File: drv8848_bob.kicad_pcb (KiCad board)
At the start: 2 copper layers, 21 x 80 mm, 21 parts, among them J1 Conn_01x04_Female, J2 Conn_01x24, J3 Conn_01x04_Female, J4 Conn_01x04_Female, J5 Conn_01x04_Female, U1 DRV8848, U2 DRV8848, U3 DRV8848, U4 DRV8848

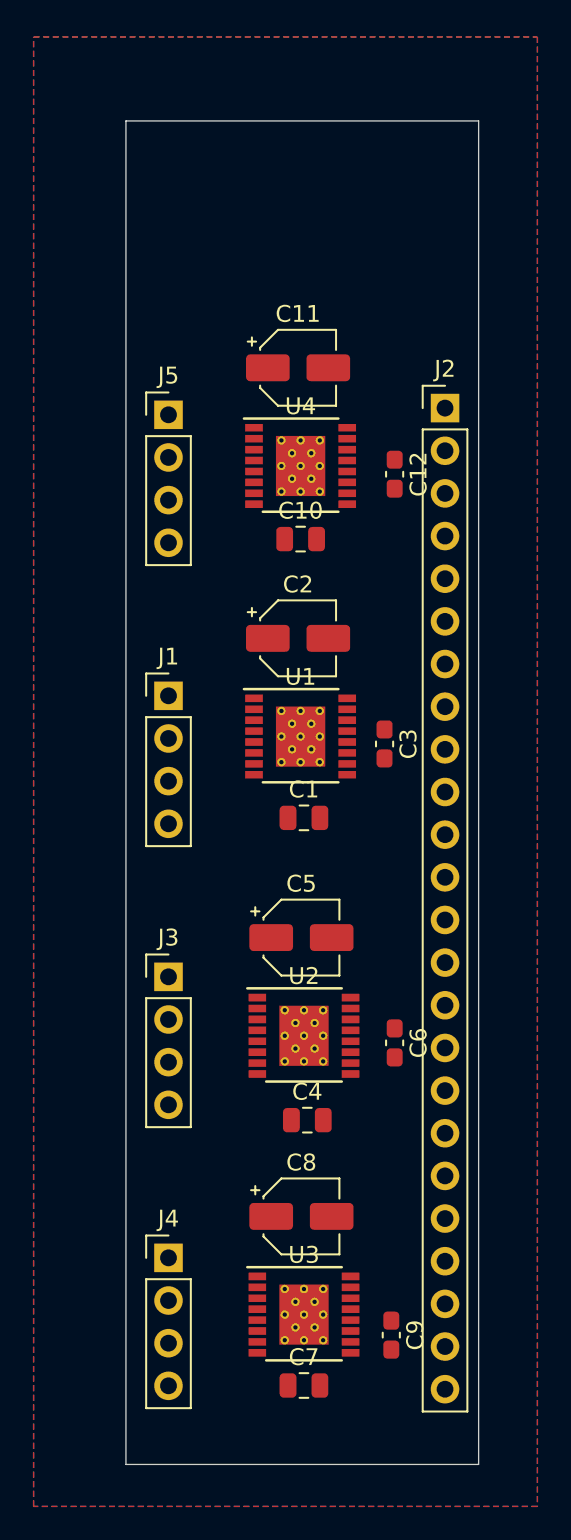
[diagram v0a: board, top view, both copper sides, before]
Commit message: finalish
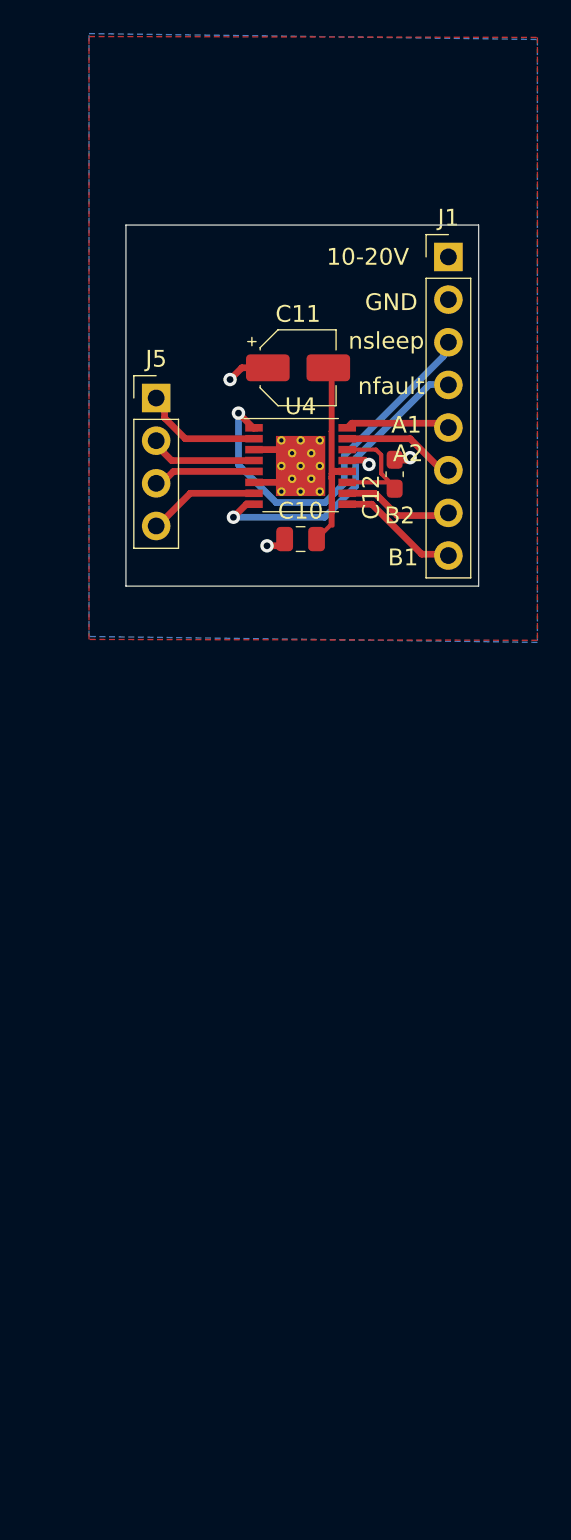
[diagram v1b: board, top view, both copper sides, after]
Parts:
- removed C1, C4, C7: 0.1uF, Capacitor_SMD:C_0805_2012Metric
- removed C2, C5, C8: 10uF, Capacitor_SMD:CP_Elec_4x5.4
- removed C3, C6, C9: 2.2uF, Capacitor_SMD:C_0603_1608Metric_Pad1.08x0.95mm_HandSolder
- removed J2: Conn_01x24, Connector_PinHeader_2.54mm:PinHeader_1x24_P2.54mm_Vertical
- removed J3, J4: Conn_01x04_Female, Connector_PinHeader_2.54mm:PinHeader_1x04_P2.54mm_Vertical
- removed U1, U2, U3: DRV8848, tachi:TSSOP-16-1EP_4.4x5mm_P0.65mm
- J1: value Conn_01x04_Female -> Conn_01x08; footprint Connector_PinHeader_2.54mm:PinHeader_1x04_P2.54mm_Vertical -> Connector_PinHeader_2.54mm:PinHeader_1x08_P2.54mm_Vertical
- moved J1 31.0 mm to (137.2, 63.1)
- moved J5 1.24 mm to (119.8, 71.5)
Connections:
- J1 pad 1: /ch1/A1 -> +12V
- J1 pad 2: /ch1/A2 -> GND
- J1 pad 3: /ch1/B2 -> nsleep[0]
- J1 pad 4: /ch1/B1 -> nfault[0]
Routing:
- net +12V: track 0.00 -> 23.4 mm
- net nsleep[0]: track 0.00 -> 23.2 mm, vias 0 -> 1
- net nfault[0]: track 0.00 -> 18.2 mm, vias 0 -> 1
- net GND: track 0.00 -> 10.9 mm, vias 0 -> 4
- net Net-(C12-Pad2): track 0.00 -> 7.48 mm
- net B1IN[0]: track 0.00 -> 7.46 mm
- net A2IN[0]: track 0.00 -> 7.07 mm
- net /sheet604C2040/A1: track 0.00 -> 7.03 mm
- net /sheet604C2040/B1: track 0.00 -> 6.81 mm
- net B2IN[0]: track 0.00 -> 6.72 mm
- net /sheet604C2040/A2: track 0.00 -> 6.35 mm
- net /sheet604C2040/B2: track 0.00 -> 6.25 mm
- net A1IN[0]: track 0.00 -> 5.84 mm
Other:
- board size 21 x 80 mm -> 21 x 21.5 mm
- board text added: "10-20V"
- board text added: "A1"
- board text added: "A2"
- board text added: "B1"
- board text added: "B2"
- board text added: "GND"
- board text added: "nfault"
- board text added: "nsleep"
